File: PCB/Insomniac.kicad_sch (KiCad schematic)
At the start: 6 parts, among them J1 PCB_USB, U1 CH32V003JxMx, U2 AP2112K-3.3

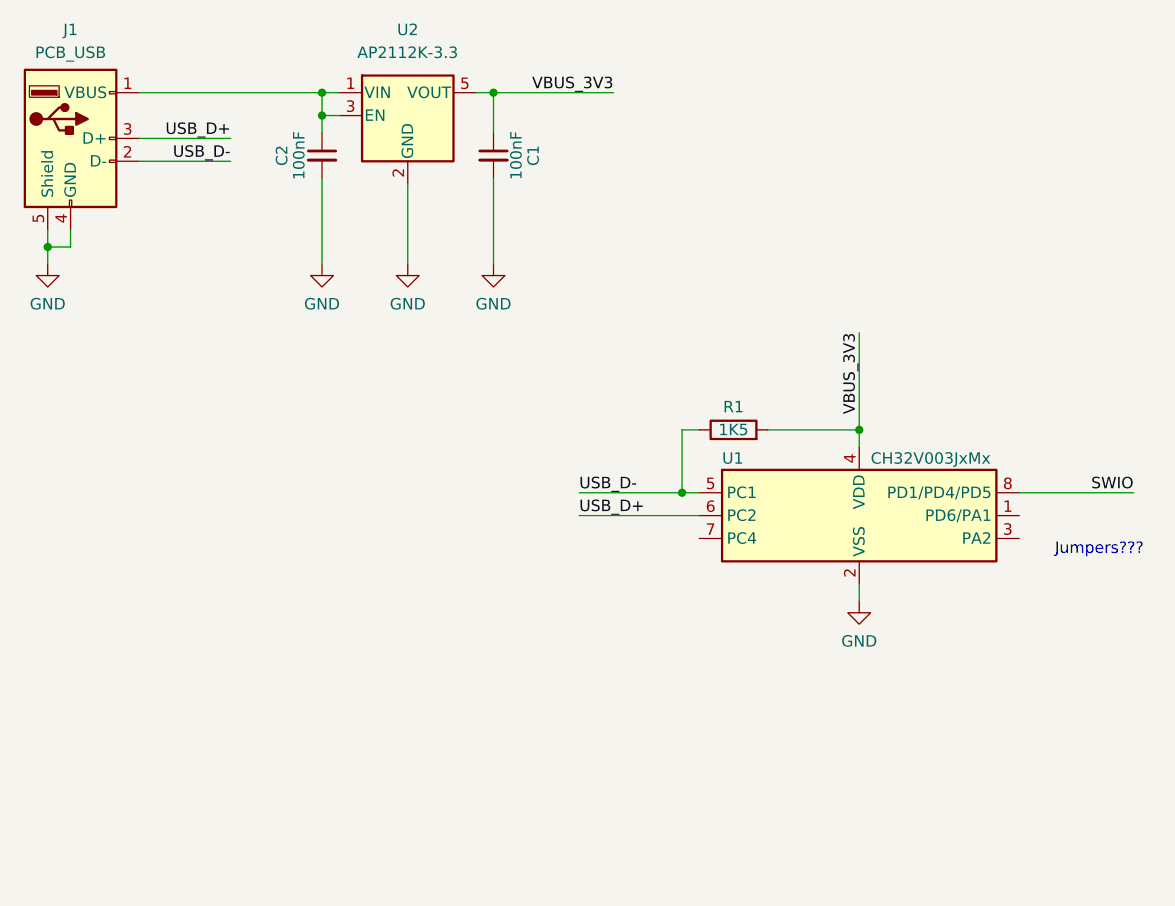
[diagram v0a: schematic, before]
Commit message: PCB Finished
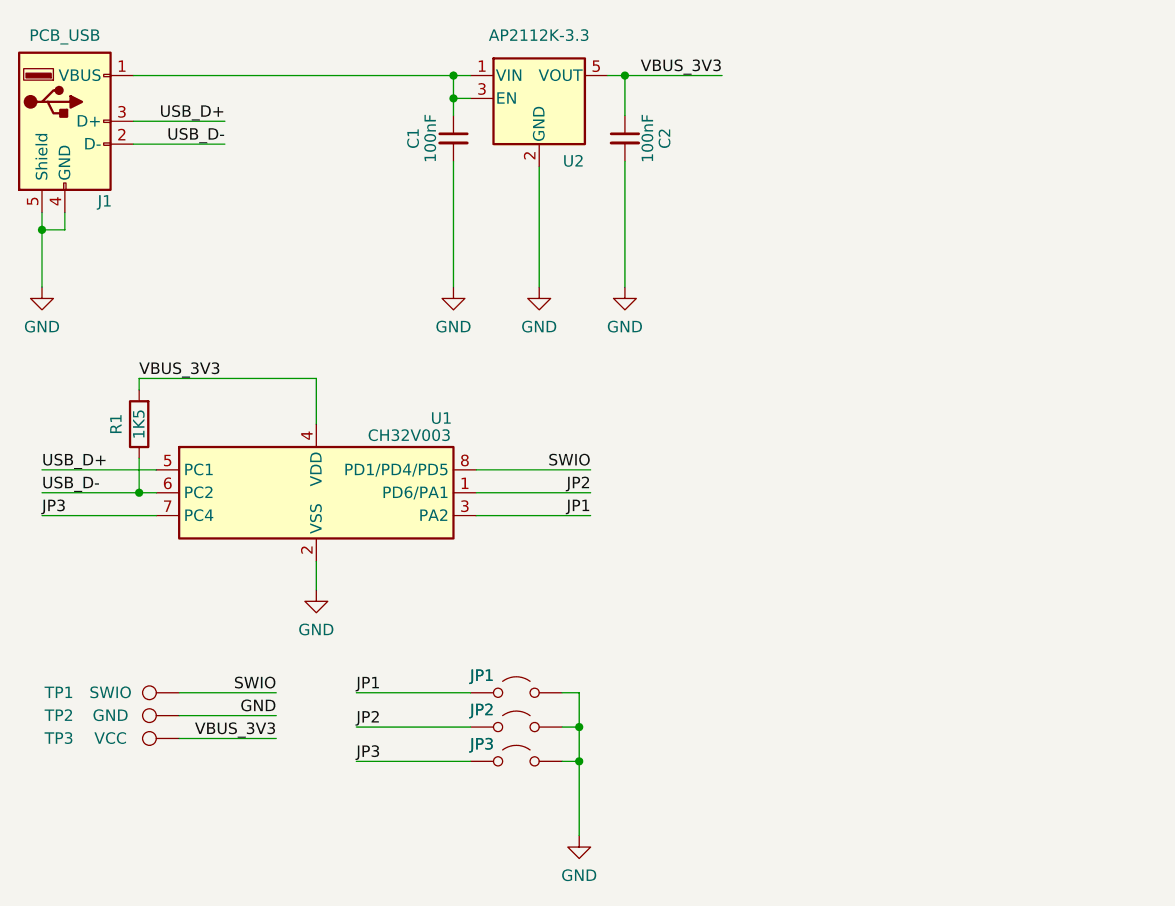
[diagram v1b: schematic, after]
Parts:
- added JP1: JP1, Jumper:SolderJumper-2_P1.3mm_Open_RoundedPad1.0x1.5mm, symbol Jumper:Jumper_2_Open
- added JP2: JP2, Jumper:SolderJumper-2_P1.3mm_Open_RoundedPad1.0x1.5mm, symbol Jumper:Jumper_2_Open
- added JP3: JP3, Jumper:SolderJumper-2_P1.3mm_Open_RoundedPad1.0x1.5mm, symbol Jumper:Jumper_2_Open
- added TP1: SWIO, TestPoint:TestPoint_Pad_D1.0mm, symbol Connector:TestPoint
- added TP2: GND, TestPoint:TestPoint_Pad_D1.0mm, symbol Connector:TestPoint
- added TP3: VCC, TestPoint:TestPoint_Pad_D1.0mm, symbol Connector:TestPoint
- C1: renamed from C2; footprint (none) -> Capacitor_SMD:C_0603_1608Metric_Pad1.08x0.95mm_HandSolder
- C2: renamed from C1; footprint (none) -> Capacitor_SMD:C_0603_1608Metric_Pad1.08x0.95mm_HandSolder
- J1: footprint (none) -> Footprints:PCB_USB_A
- R1: footprint (none) -> Resistor_SMD:R_0603_1608Metric_Pad0.98x0.95mm_HandSolder
- U1: value CH32V003JxMx -> CH32V003
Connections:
- net GND: now also JP1.2 (B), JP2.2 (B), JP3.2 (B), TP2.1
- net SWIO: now also TP1.1
- net USB_D+: now also U1.5 (PC1); no longer U1.6 (PC2)
- net USB_D-: now also U1.6 (PC2); no longer U1.5 (PC1)
- net VBUS_3V3: now also TP3.1
- net JP2: now reaches U1.1 (PD6/PA1)
- net JP2: now also JP2.1 (A)
- net JP1: now reaches U1.3 (PA2)
- net JP1: now also JP1.1 (A)
- net JP3: now reaches U1.7 (PC4)
- net JP3: now also JP3.1 (A)
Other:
- note removed: "Jumpers???"
- moved on the sheet: C1, C2, J1, R1, U1, U2
